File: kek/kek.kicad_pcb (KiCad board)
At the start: 2 copper layers, 65 x 85 mm, 26 parts, among them X1 B3P-VH

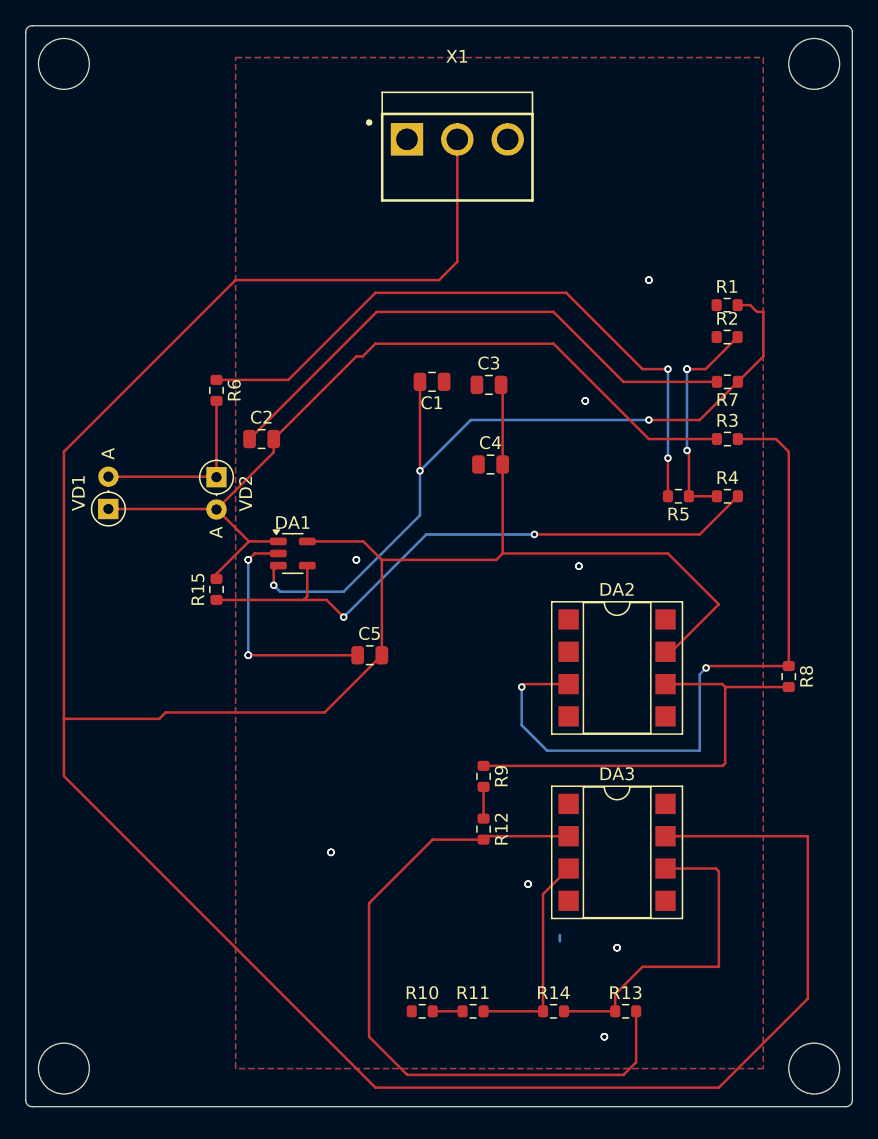
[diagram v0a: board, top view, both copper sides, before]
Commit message: new files
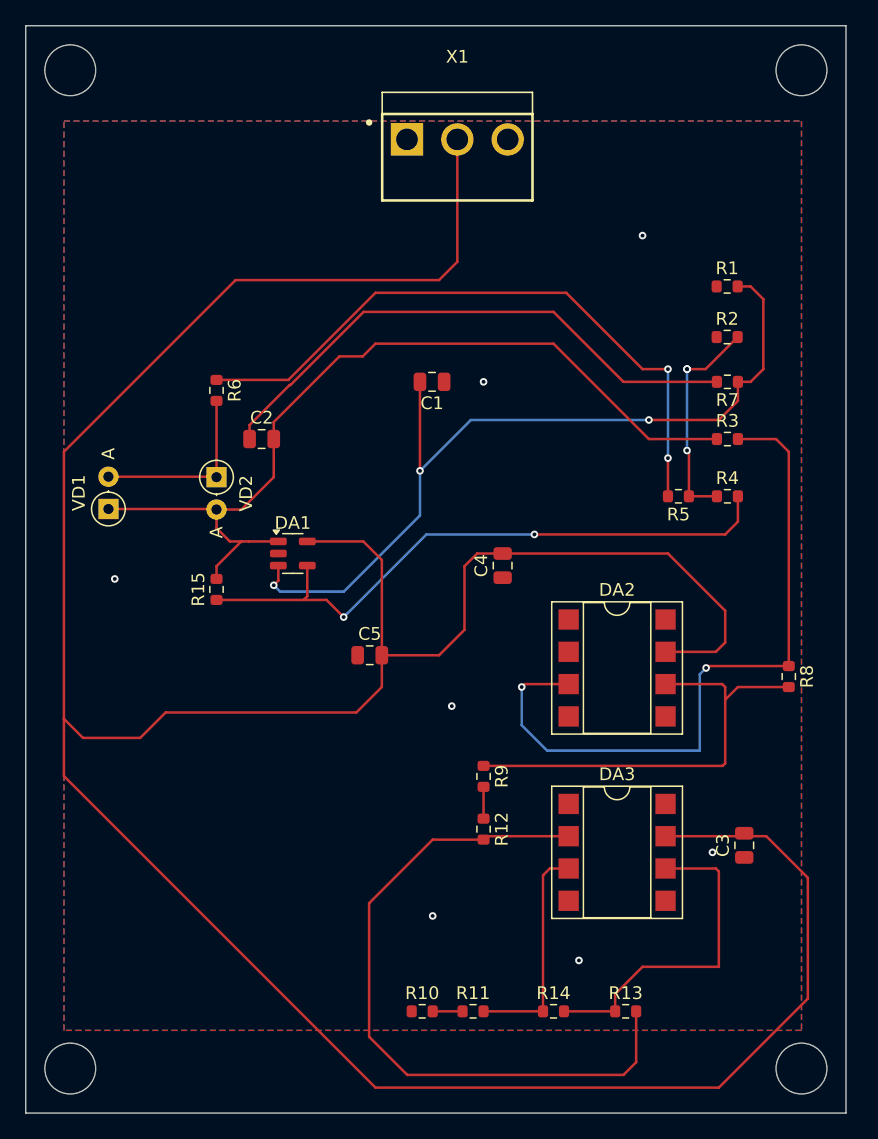
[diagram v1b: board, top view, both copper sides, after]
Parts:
- moved C3 41.4 mm to (156.5, 124.5), turned to 90 degrees
- moved C4 8.01 mm to (137.5, 102.5), turned to 90 degrees
- moved R1 1.47 mm to (155.2, 80.5)
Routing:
- net Earth: track 18.7 -> 0.00 mm, vias 20 -> 7
- net +5V: track 256.2 -> 252.2 mm
- net Net-(DA1-IN+): track 62.9 -> 65.5 mm
- net /OUT1: track 66.9 -> 69.5 mm
- net Net-(DA1-IN-): track 48.7 -> 49.8 mm
- net Net-(DA3-IN-): track 16.7 -> 17.6 mm
- net Net-(C2-Pad1): track 43.2 -> 43.8 mm
- net (no net): track 0.50 -> 0.00 mm
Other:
- board size 65 x 85 mm -> 64.5 x 85.5 mm
